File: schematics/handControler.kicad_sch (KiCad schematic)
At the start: 12 parts, among them SW1 SW_MEC_5G, SW1 balast, SW2 revers, SW2 switch display

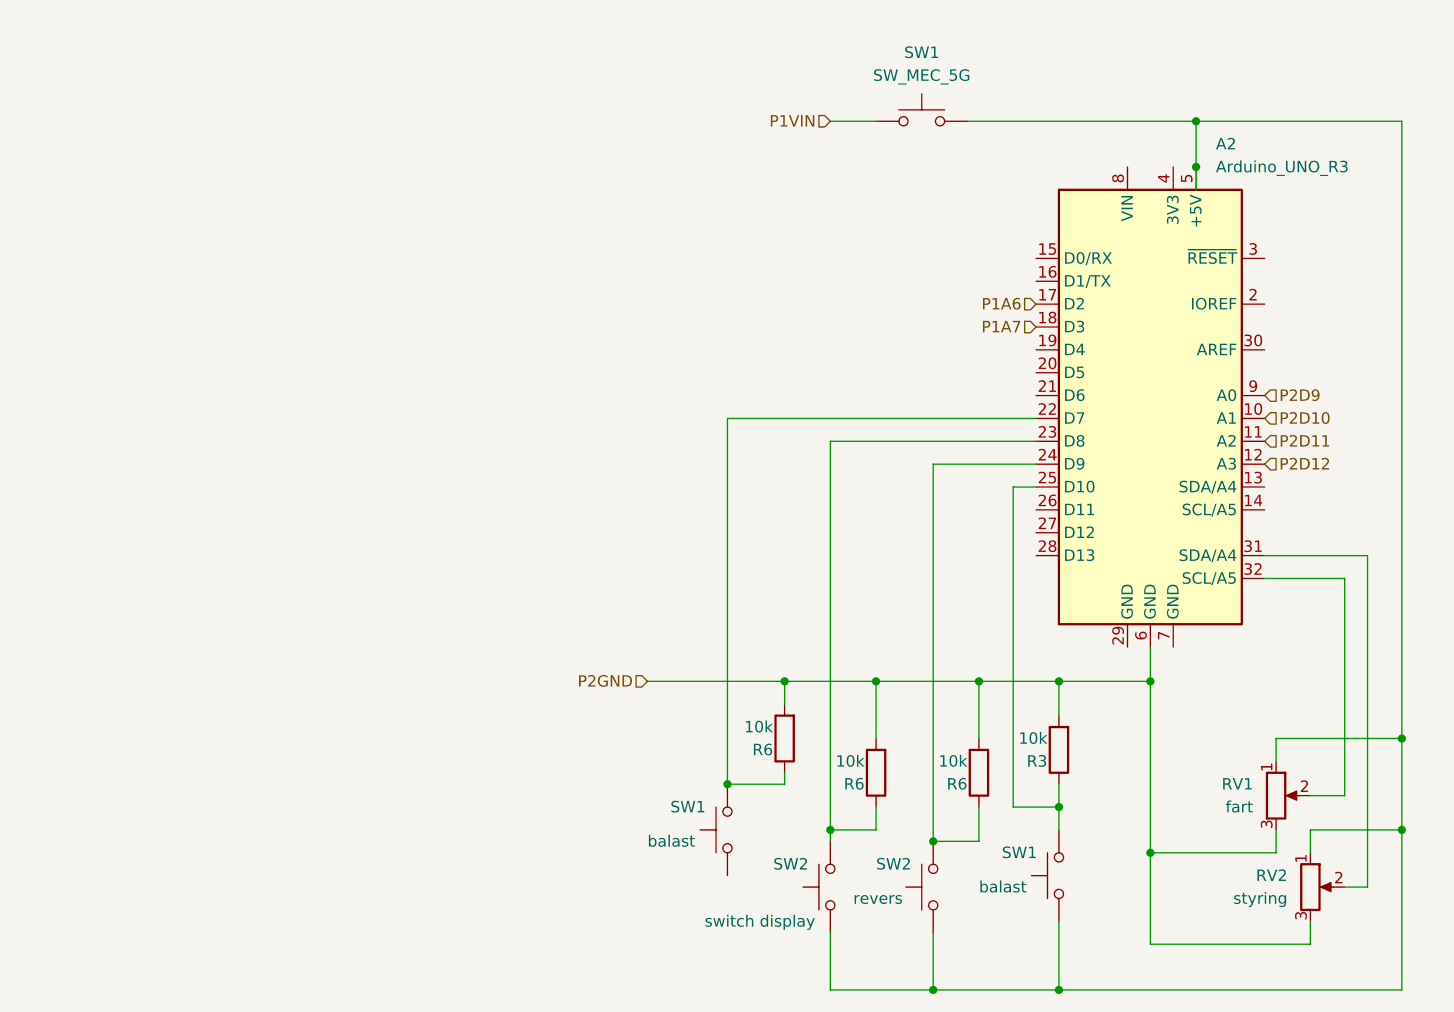
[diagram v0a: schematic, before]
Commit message: updated handcontroler
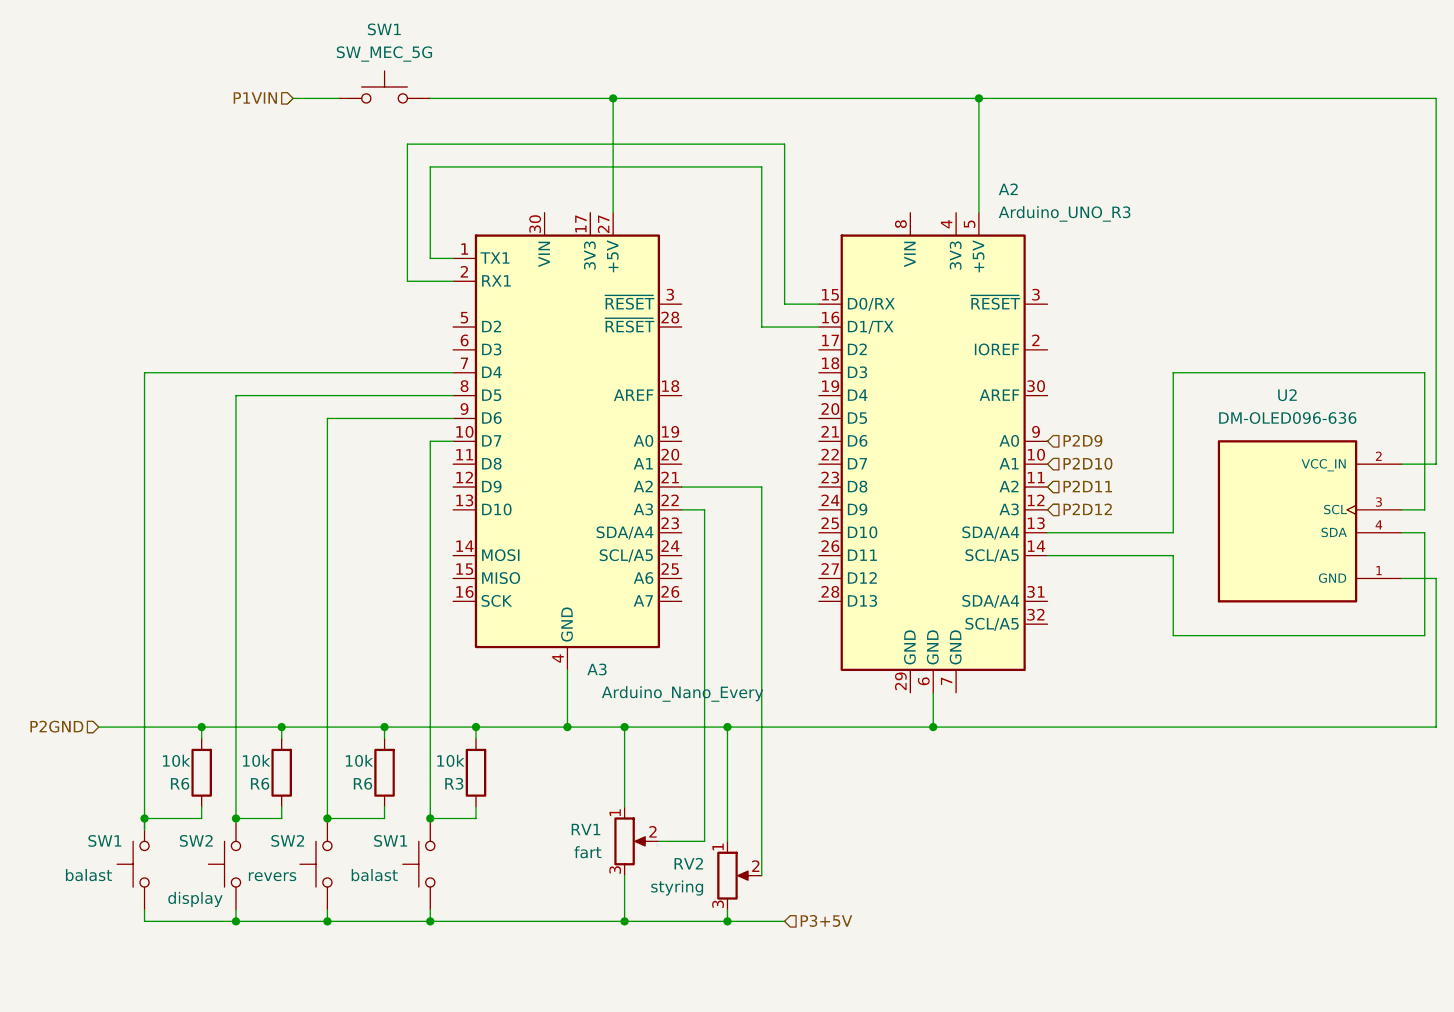
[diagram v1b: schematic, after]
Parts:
- added A3: Arduino_Nano_Every, Module:Arduino_Nano, symbol MCU_Module:Arduino_Nano_Every
- added U2: DM-OLED096-636, DM-OLED096-636:MODULE_DM-OLED096-636, symbol DM-OLED096-636:DM-OLED096-636
- SW2: value switch display -> display
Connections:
- net P2GND: now also RV1.1, RV2.1, A3.29 (GND), A3.4 (GND), U2.1 (GND); no longer RV1.3, RV2.3
- net at R6.1, SW2.2: now also A3.9 (D6); no longer A2.24 (D9)
- net at R3.1, SW1.2: now also A3.10 (D7); no longer A2.25 (D10)
- net P3+5V: now reaches SW1.1
- net P3+5V: now also RV1.3, RV2.3, SW1.1, SW2.1, SW2.1
- net at R6.1, SW1.2: now also A3.7 (D4); no longer A2.22 (D7)
- net at R6.1, SW2.2: now also A3.8 (D5); no longer A2.23 (D8)
- net at A2.13 (SDA/A4): now also U2.3 (SCL)
- net at A2.14 (SCL/A5): now also U2.4 (SDA)
- net at A2.15 (D0/RX): now also A3.2 (RX1)
- net at A2.16 (D1/TX): now also A3.1 (TX1)
- net at A2.31 (SDA/A4): no longer RV2.2
- net at A2.32 (SCL/A5): no longer RV1.2
- net P1A6: no longer names the net of A2.17 (D2)
- net P1A7: no longer names the net of A2.18 (D3)
- new net: A2.5 (+5V), A3.27 (+5V), SW1.3 (B), SW1.4 (B), U2.2 (VCC_IN)
- new net: A3.21 (A2), RV2.2
- new net: A3.22 (A3), RV1.2
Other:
- moved on the sheet: R3, R6, SW1, SW2
